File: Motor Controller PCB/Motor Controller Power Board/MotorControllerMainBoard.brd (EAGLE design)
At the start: 60 x 100 mm, 52 parts, among them U1 CDBA340L-G

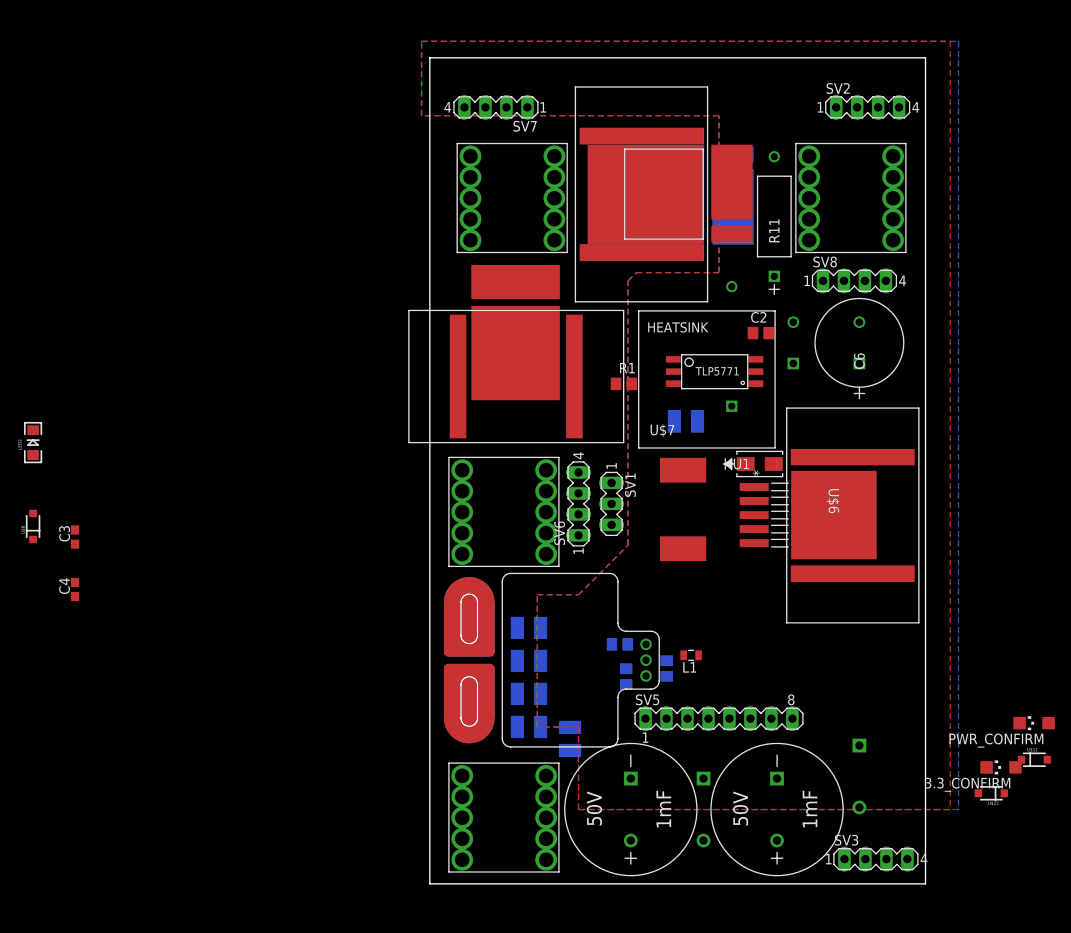
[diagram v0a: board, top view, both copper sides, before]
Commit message: Made a layout, need labels
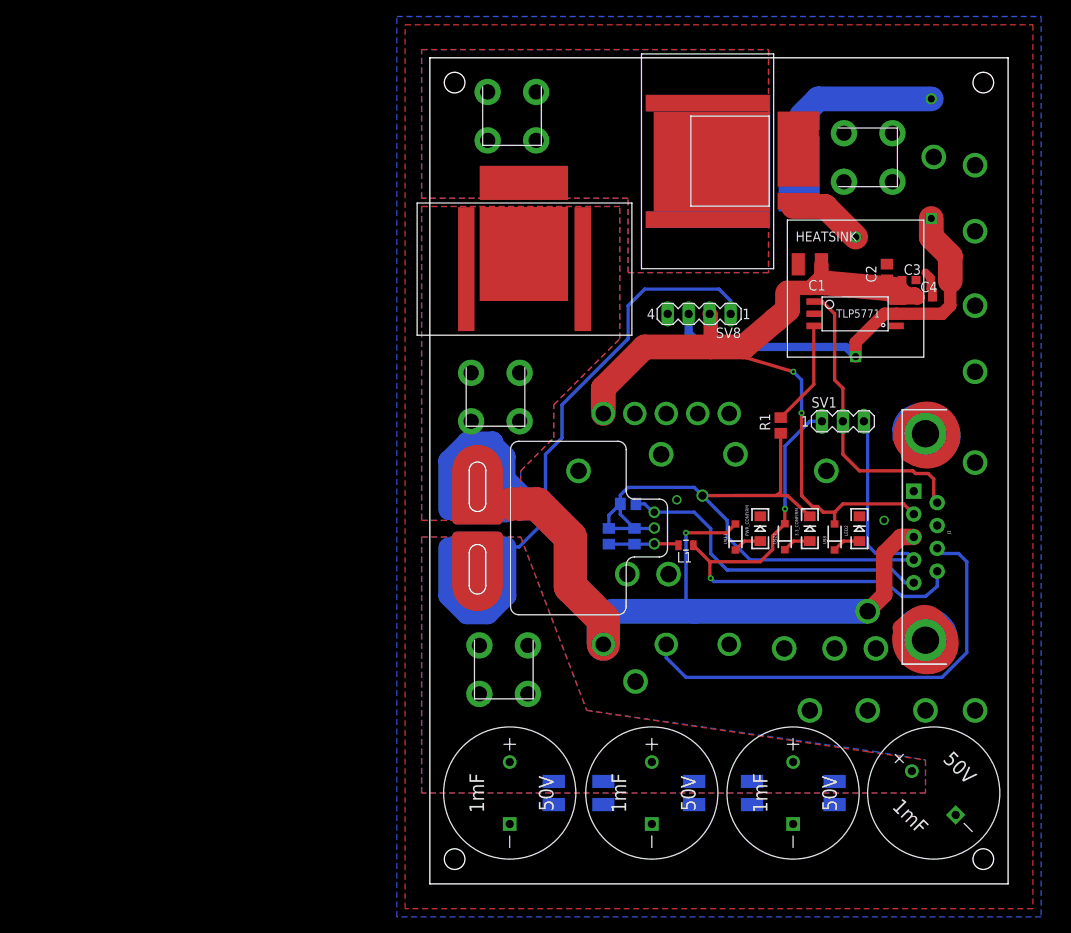
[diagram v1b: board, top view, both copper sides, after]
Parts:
- removed C5, C6: EEUFR1H221B, MotorControllerEagleLibrary:CAP_PAN_10X16
- removed SV2, SV3, SV6, SV7: (no value), con-lstb:MA04-1
- removed SV5: (no value), con-lstb:MA08-1
- removed U$24: DA-T263-101E, MotorControllerEagleLibrary:DA-T263-101E
- removed U$7: 100uH, MotorControllerEagleLibrary:INDUCTOR_SMD_FOOTPRINT
- removed U1: CDBA340L-G, MotorControllerEagleLibrary:CDBA-G
- added J1: (no value), SparkFun-Connectors:DB9
- 3.3_CONFIRM, PWR_CONFIRM: device led:CHIPLED_1206 -> SparkFun-LED:LED-1206
- U$12, U$14, U$15, U$16: value 732-3204-ND_CONNECTOR -> 74650073R; device Connector 732-3204:732-3204-ND -> MotorControllerEagleLibrary:74650073R
- U$6: value TL2575HV-15IKTTR -> KHHD004A2B; device MotorControllerEagleLibrary:KTT5_6P22X6P86 -> MotorControllerEagleLibrary:KHHD004A2B
- moved C4 108.9 mm to (60.0, 71.0), turned to 0 degrees
- moved C3 105.6 mm to (58.0, 73.1), turned to 0 degrees
- moved LED2 100.6 mm to (52.0, 43.0)
- moved U$8 97.0 mm to (49.0, 42.0)
- moved U$12 82.0 mm to (7.00, 90.0), turned to 0 degrees
- moved U$15 61.7 mm to (56.0, 85.0)
- moved U$16 60.1 mm to (6.00, 23.0), turned to 0 degrees
- moved U$14 53.3 mm to (5.00, 56.0), turned to 0 degrees
- moved U$11 45.1 mm to (37.0, 42.0), turned to 90 degrees
- moved PWR_CONFIRM 40.7 mm to (40.0, 43.0)
- moved U$22 39.9 mm to (43.0, 42.0), turned to 90 degrees
- moved 3.3_CONFIRM 37.0 mm to (46.0, 43.0)
- moved C38 32.7 mm to (49.0, 11.0), turned to 270 degrees
- moved U$6 32.0 mm to (21.0, 29.0), flipped to the bottom, turned to 90 degrees
- moved C40 31.4 mm to (39.0, 11.0), turned to 270 degrees
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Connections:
- removed net N$1: U$6.2, U$7.1, U1.1
- removed net POWER_INPUT(+): U$9.PIN5
- new net ENABLE_12V: J1.8, U$6.ON/OFF
- new net N$11: U$6.SENSE+
- new net N$5: U$6.SENSE-
- new net N$8: U$6.TRIM
- net 12V_POWER_REGULATED: now also J1.2, U$6.VO+; no longer C5.1, C6.1, U$6.4, U$7.2
- net 3.3V_ISOLATED: now also J1.1, J1.9; no longer SV5.5, SV6.1
- net CURRENT_SENSOR_OUTPUT: now also J1.5; no longer SV5.7
- net GND: now also J1.7, U$15.P$1, U$15.P$2, U$15.P$3, U$15.P$4, U$6.VI-, U$6.VO-; no longer C5.2, C6.2, SV5.3, SV5.4, U$14.P$1, U$14.P$10, U$14.P$2, U$14.P$3, U$14.P$4, U$14.P$5, U$14.P$6, U$14.P$7, U$14.P$8, U$14.P$9, U$24.GND, U$24.GND2\, U$6.3, U$6.5, U$6.6, U1.2
- net GND_ISOLATED: now also J1.4; no longer SV5.6, SV5.8, SV6.2, SV6.4
- net INPUT_POWER(+): now also J1.3, U$14.P$1, U$14.P$2, U$14.P$3, U$14.P$4, U$6.VI+, U$9.PIN4; no longer C36.1, C37.1, C38.1, C39.1, C40.1, SV5.1, SV5.2, U$10.POSITIVE, U$12.P$1, U$12.P$10, U$12.P$2, U$12.P$3, U$12.P$4, U$12.P$5, U$12.P$6, U$12.P$7, U$12.P$8, U$12.P$9, U$13.POSITIVE, U$18.POSITIVE, U$19.POSITIVE
- net MOTOR_OUTPUT_(+): now also C36.1, C37.1, C38.1, C39.1, C40.1, U$10.POSITIVE, U$13.POSITIVE, U$16.P$1, U$16.P$2, U$16.P$3, U$16.P$4, U$18.POSITIVE, U$19.POSITIVE, U$9.PIN5; no longer U$15.P$1, U$15.P$10, U$15.P$2, U$15.P$3, U$15.P$4, U$15.P$5, U$15.P$6, U$15.P$7, U$15.P$8, U$15.P$9, U$6.1, U$9.PIN4
- net MOTOR_OUTPUT_(--): now also U$12.P$1, U$12.P$2, U$12.P$3, U$12.P$4; no longer U$16.P$1, U$16.P$10, U$16.P$2, U$16.P$3, U$16.P$4, U$16.P$5, U$16.P$6, U$16.P$7, U$16.P$8, U$16.P$9
- net TEENSY_FET_DRIVER_SIGNAL: now also J1.6, U$17.1.ANODE; no longer SV6.3
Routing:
- net INPUT_POWER(+): track 0.00 -> 131.8 mm, vias 0 -> 2
- net 12V_POWER_REGULATED: track 0.00 -> 103.0 mm, vias 0 -> 2
- net GND_ISOLATED: track 0.00 -> 97.9 mm, vias 0 -> 1
- net MOTOR_OUTPUT_(+): track 0.00 -> 72.1 mm
- net 3.3V_ISOLATED: track 0.00 -> 62.4 mm, vias 0 -> 2
- net GND: track 0.00 -> 56.9 mm, vias 0 -> 22
- net ENABLE_12V: track 0.00 -> 55.5 mm
- net FET_DRIVER_SIGNAL: track 0.00 -> 50.3 mm
- net CURRENT_SENSOR_OUTPUT: track 0.00 -> 39.4 mm
- net TEENSY_FET_DRIVER_SIGNAL: track 0.00 -> 35.8 mm
- net N$10: track 0.00 -> 17.4 mm
- net N$7: track 0.00 -> 12.8 mm
- net N$2: track 0.00 -> 9.98 mm
- net N$6: track 0.00 -> 8.52 mm
- net N$14: track 0.00 -> 3.47 mm
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- added copper zone on layer 1, net INPUT_POWER(+)
- added copper zone on layer 16, net INPUT_POWER(+)
- added copper zone on layer 1, net MOTOR_OUTPUT_(+)
- added copper zone on layer 16, net MOTOR_OUTPUT_(+)
- added copper zone on layer 1, net MOTOR_OUTPUT_(--)
- added copper zone on layer 16, net MOTOR_OUTPUT_(--)
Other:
- board size 60 x 100 mm -> 70 x 100 mm
